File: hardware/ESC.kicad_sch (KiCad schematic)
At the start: 36 parts, among them Q1 DOY180N03T, Q2 DOY180N03T, Q3 DOY180N03T, Q4 DOY180N03T, Q5 DOY180N03T, Q6 DOY180N03T, U2 AT32F421G8U7, U3 NSG2065Q

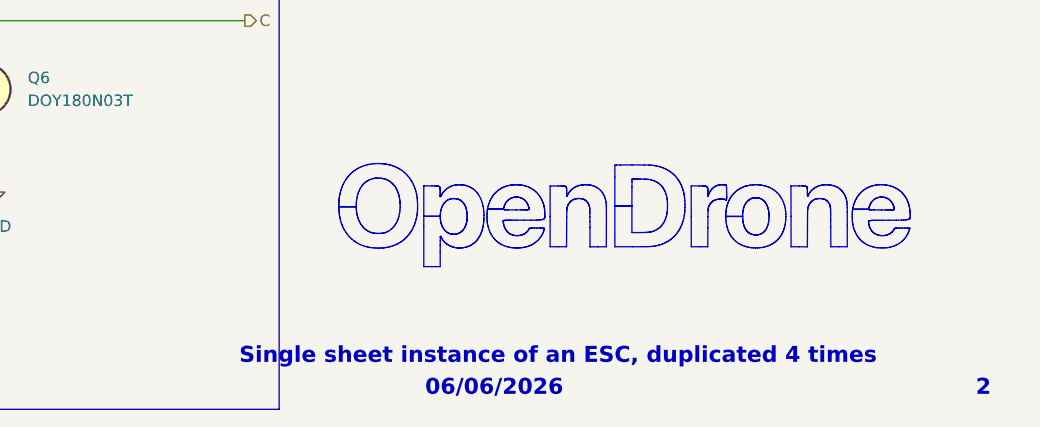
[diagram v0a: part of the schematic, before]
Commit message: SFT naming update
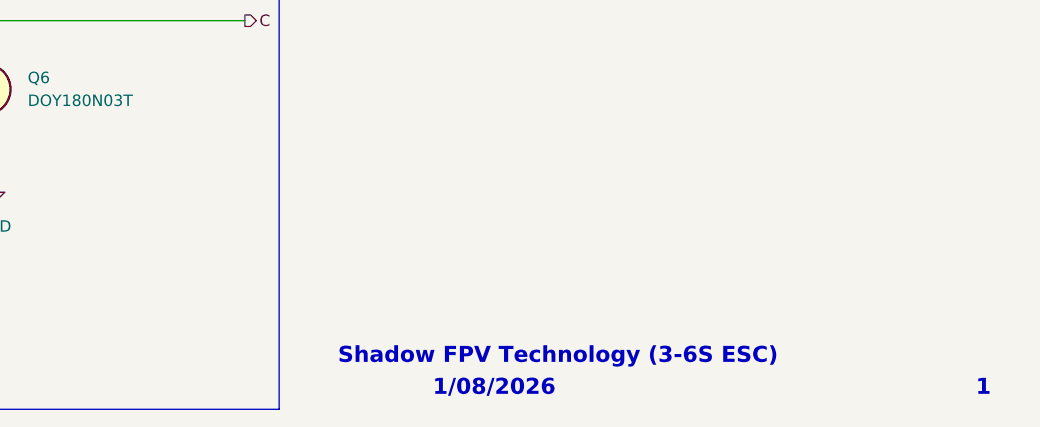
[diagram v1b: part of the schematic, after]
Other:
- note added: "1"
- note added: "1/08/2026"
- note added: "Shadow FPV Technology (3-6S ESC)"
- note removed: "06/06/2026"
- note removed: "2"
- note removed: "Single sheet instance of an ESC, duplicated 4 times"
